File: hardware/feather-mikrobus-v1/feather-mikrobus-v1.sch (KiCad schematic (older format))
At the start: 25 parts, among them J1 Adafruit_Feather_socket_heade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, J2 Adafruit_Feather_socket_heade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, J3 mikroBUS_socket_header_left_p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, J4 mikroBUS_socket_header_right_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, SW1 C_and_K_JS102011SAQN, SW2 C_and_K_KMR421GULCLFS, SW3 C_and_K_KMR421GULCLFS

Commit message: WIP
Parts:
- C1: symbol Flying_Camp_Design:Murata_GRM188R72A104KA35D -> feather-mikrobus-v1-rescue:Murata_GRM188R72A104KA35D-Flying_Camp_Design
- D1, D2: symbol Flying_Camp_Design:Lite-On_LTST-C193KGKT-5A -> feather-mikrobus-v1-rescue:Lite-On_LTST-C193KGKT-5A-Flying_Camp_Design
- FID1, FID2, FID3: symbol Flying_Camp_Design:Fiducial_1mm_Mask2mm -> feather-mikrobus-v1-rescue:Fiducial_1mm_Mask2mm-Flying_Camp_Design
- J1: symbol Flying_Camp_Design:Adafruit_Feather_socket_header_left_pth -> feather-mikrobus-v1-rescue:Adafruit_Feather_socket_header_left_pth-Flying_Camp_Design
- J2: symbol Flying_Camp_Design:Adafruit_Feather_socket_header_right_pth -> feather-mikrobus-v1-rescue:Adafruit_Feather_socket_header_right_pth-Flying_Camp_Design
- J3: symbol Flying_Camp_Design:mikroBUS_socket_header_left_pth -> feather-mikrobus-v1-rescue:mikroBUS_socket_header_left_pth-Flying_Camp_Design
- J4: symbol Flying_Camp_Design:mikroBUS_socket_header_right_pth -> feather-mikrobus-v1-rescue:mikroBUS_socket_header_right_pth-Flying_Camp_Design
- LOGO1: symbol Flying_Camp_Design:mikroBUS-Logo_11.9x4.1mm_SilkScreen -> feather-mikrobus-v1-rescue:mikroBUS-Logo_11.9x4.1mm_SilkScreen-Flying_Camp_Design
- LOGO2: symbol Flying_Camp_Design:Flying_Camp_Design_logo_7.35x11mm_silkscreen -> feather-mikrobus-v1-rescue:Flying_Camp_Design_logo_7.35x11mm_silkscreen-Flying_Camp_Design
- LOGO3: symbol Flying_Camp_Design:Adafruit_Feather_logo_13.87x6.33mm_silkscreen -> feather-mikrobus-v1-rescue:Adafruit_Feather_logo_13.87x6.33mm_silkscreen-Flying_Camp_Design
- MH1: symbol Flying_Camp_Design:Adafruit_Feather_socket_mounting_holes -> feather-mikrobus-v1-rescue:Adafruit_Feather_socket_mounting_holes-Flying_Camp_Design
- R1: symbol Flying_Camp_Design:Yageo_RC0603JR-071KL -> feather-mikrobus-v1-rescue:Yageo_RC0603JR-071KL-Flying_Camp_Design
- R2, R8: symbol Flying_Camp_Design:Yageo_RC0603JR-07330RL -> feather-mikrobus-v1-rescue:Yageo_RC0603JR-07330RL-Flying_Camp_Design
- R3, R4: symbol Flying_Camp_Design:Yageo_RC0603JR-074K7L -> feather-mikrobus-v1-rescue:Yageo_RC0603JR-074K7L-Flying_Camp_Design
- R5: symbol Flying_Camp_Design:Yageo_RC0603JR-070RL -> feather-mikrobus-v1-rescue:Yageo_RC0603JR-070RL-Flying_Camp_Design
- R6: symbol Flying_Camp_Design:Yageo_RC0603JR-0710KL -> feather-mikrobus-v1-rescue:Yageo_RC0603JR-0710KL-Flying_Camp_Design
- R7: symbol Flying_Camp_Design:Yageo_RC0603JR-07100RL -> feather-mikrobus-v1-rescue:Yageo_RC0603JR-07100RL-Flying_Camp_Design
- SW1: symbol Flying_Camp_Design:C_and_K_JS102011SAQN -> feather-mikrobus-v1-rescue:C_and_K_JS102011SAQN-Flying_Camp_Design
- SW2, SW3: symbol Flying_Camp_Design:C_and_K_KMR421GULCLFS -> feather-mikrobus-v1-rescue:C_and_K_KMR421GULCLFS-Flying_Camp_Design
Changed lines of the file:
@@
 3V3_LED_R
 $Comp
-L Flying_Camp_Design:C_and_K_KMR421GULCLFS SW3
+L feather-mikrobus-v1-rescue:C_and_K_KMR421GULCLFS-Flying_Camp_Design SW3
 U 1 1 5E5A44D1
 P 8800 4800
@@
 $EndComp
 $Comp
-L Flying_Camp_Design:Yageo_RC0603JR-074K7L R4
+L feather-mikrobus-v1-rescue:Yageo_RC0603JR-074K7L-Flying_Camp_Design R4
 U 1 1 5E4ACFB9
 P 7500 2800
@@
 $EndComp
 $Comp
-L Flying_Camp_Design:Yageo_RC0603JR-074K7L R3
+L feather-mikrobus-v1-rescue:Yageo_RC0603JR-074K7L-Flying_Camp_Design R3
 U 1 1 5E4AC677
 P 7100 2800
@@
 $EndComp
 $Comp
-L Flying_Camp_Design:C_and_K_JS102011SAQN SW1
+L feather-mikrobus-v1-rescue:C_and_K_JS102011SAQN-Flying_Camp_Design SW1
 U 1 1 5E49923D
 P 8000 2100
@@
 $EndComp
 $Comp
-L Flying_Camp_Design:+3.3V #PWR08
+L feather-mikrobus-v1-rescue:+3.3V-Flying_Camp_Design #PWR08
 U 1 1 5E401342
 P 7500 2600
@@
 $EndComp
 $Comp
-L Flying_Camp_Design:+3.3V #PWR07
+L feather-mikrobus-v1-rescue:+3.3V-Flying_Camp_Design #PWR07
 U 1 1 5E4009E4
 P 7100 2600
@@
 $EndComp
 $Comp
-L Flying_Camp_Design:+3.3V #PWR02
+L feather-mikrobus-v1-rescue:+3.3V-Flying_Camp_Design #PWR02
 U 1 1 5E3DD319
 P 4800 1300
@@
 $EndComp
 $Comp
-L Flying_Camp_Design:Adafruit_Feather_socket_mounting_holes MH1
+L feather-mikrobus-v1-rescue:Adafruit_Feather_socket_mounting_holes-Flying_Camp_Design MH1
 U 1 1 5E3B84FB
 P 5600 1700
@@
 $EndComp
 $Comp
-L Flying_Camp_Design:Adafruit_Feather_socket_header_left_pth J1
+L feather-mikrobus-v1-rescue:Adafruit_Feather_socket_header_left_pth-Flying_Camp_Design J1
 U 1 1 5E3B727D
 P 5200 2300
@@
 $EndComp
 $Comp
-L Flying_Camp_Design:Adafruit_Feather_socket_header_right_pth J2
+L feather-mikrobus-v1-rescue:Adafruit_Feather_socket_header_right_pth-Flying_Camp_Design J2
 U 1 1 5E3B67CD
 P 5600 2500
@@
 $EndComp
 $Comp
-L Flying_Camp_Design:Adafruit_Feather_logo_13.87x6.33mm_silkscreen LOGO3
+L feather-mikrobus-v1-rescue:Adafruit_Feather_logo_13.87x6.33mm_silkscreen-Flying_Camp_Design LOGO3
 U 1 1 5E42FCDA
 P 5400 1300
@@
 $EndComp
 $Comp
-L Flying_Camp_Design:C_and_K_KMR421GULCLFS SW2
+L feather-mikrobus-v1-rescue:C_and_K_KMR421GULCLFS-Flying_Camp_Design SW2
 U 1 1 5E4768B4
 P 2900 2600
@@
 $EndComp
 $Comp
-L Flying_Camp_Design:+3.3V #PWR0103
+L feather-mikrobus-v1-rescue:+3.3V-Flying_Camp_Design #PWR0103
 U 1 1 5E47840A
 P 2900 1800
@@
 $EndComp
 $Comp
-L Flying_Camp_Design:Yageo_RC0603JR-070RL R5
+L feather-mikrobus-v1-rescue:Yageo_RC0603JR-070RL-Flying_Camp_Design R5
 U 1 1 5E4BAA63
 P 3900 1600
@@
 $EndComp
 $Comp
-L Flying_Camp_Design:Yageo_RC0603JR-071KL R1
+L feather-mikrobus-v1-rescue:Yageo_RC0603JR-071KL-Flying_Camp_Design R1
 U 1 1 5E4237BC
 P 2900 2000
@@
 $EndComp
 $Comp
-L Flying_Camp_Design:Yageo_RC0603JR-07100RL R7
+L feather-mikrobus-v1-rescue:Yageo_RC0603JR-07100RL-Flying_Camp_Design R7
 U 1 1 5E42A109
 P 8700 2400
@@
 $EndComp
 $Comp
-L Flying_Camp_Design:+3.3V #PWR09
+L feather-mikrobus-v1-rescue:+3.3V-Flying_Camp_Design #PWR09
 U 1 1 5E3DE1B7
 P 2100 4600
@@
 $EndComp
 $Comp
-L Flying_Camp_Design:mikroBUS_socket_header_left_pth J3
+L feather-mikrobus-v1-rescue:mikroBUS_socket_header_left_pth-Flying_Camp_Design J3
 U 1 1 5E3C6EE3
 P 2500 5000
@@
 $EndComp
 $Comp
-L Flying_Camp_Design:mikroBUS_socket_header_right_pth J4
+L feather-mikrobus-v1-rescue:mikroBUS_socket_header_right_pth-Flying_Camp_Design J4
 U 1 1 5E3C7996
 P 2900 5000
@@
 $EndComp
 $Comp
-L Flying_Camp_Design:mikroBUS-Logo_11.9x4.1mm_SilkScreen LOGO1
+L feather-mikrobus-v1-rescue:mikroBUS-Logo_11.9x4.1mm_SilkScreen-Flying_Camp_Design LOGO1
 U 1 1 5E3FB24F
 P 2700 4400
@@
 $EndComp
 $Comp
-L Flying_Camp_Design:+3.3V #PWR0107
+L feather-mikrobus-v1-rescue:+3.3V-Flying_Camp_Design #PWR0107
 U 1 1 5E5B7B5B
 P 7900 4500
@@
 $EndComp
 $Comp
-L Flying_Camp_Design:Yageo_RC0603JR-0710KL R6
+L feather-mikrobus-v1-rescue:Yageo_RC0603JR-0710KL-Flying_Camp_Design R6
 U 1 1 5E425364
 P 7900 4700
@@
 $EndComp
 $Comp
-L Flying_Camp_Design:Murata_GRM188R72A104KA35D C1
+L feather-mikrobus-v1-rescue:Murata_GRM188R72A104KA35D-Flying_Camp_Design C1
 U 1 1 5E427A0D
 P 7900 5100
@@
 $EndComp
 $Comp
-L Flying_Camp_Design:Yageo_RC0603JR-07330RL R8
+L feather-mikrobus-v1-rescue:Yageo_RC0603JR-07330RL-Flying_Camp_Design R8
 U 1 1 5E49B00C
 P 6000 4700
@@
 $EndComp
 $Comp
-L Flying_Camp_Design:+3.3V #PWR0110
+L feather-mikrobus-v1-rescue:+3.3V-Flying_Camp_Design #PWR0110
 U 1 1 5E49AFEA
 P 6000 4500
@@
 $EndComp
 $Comp
-L Flying_Camp_Design:Yageo_RC0603JR-07330RL R2
+L feather-mikrobus-v1-rescue:Yageo_RC0603JR-07330RL-Flying_Camp_Design R2
 U 1 1 5E41F1AC
 P 5300 4700
@@
 $EndComp
 $Comp
-L Flying_Camp_Design:+3.3V #PWR0109
+L feather-mikrobus-v1-rescue:+3.3V-Flying_Camp_Design #PWR0109
 U 1 1 5E6244BC
 P 5300 4500
@@
 $EndComp
 $Comp
-L Flying_Camp_Design:Fiducial_1mm_Mask2mm FID3
+L feather-mikrobus-v1-rescue:Fiducial_1mm_Mask2mm-Flying_Camp_Design FID3
 U 1 1 5E3F3D03
 P 4700 7700
@@
 $EndComp
 $Comp
-L Flying_Camp_Design:Fiducial_1mm_Mask2mm FID2
+L feather-mikrobus-v1-rescue:Fiducial_1mm_Mask2mm-Flying_Camp_Design FID2
 U 1 1 5E3F3A33
 P 4700 7500
@@
 $EndComp
 $Comp
-L Flying_Camp_Design:Fiducial_1mm_Mask2mm FID1
+L feather-mikrobus-v1-rescue:Fiducial_1mm_Mask2mm-Flying_Camp_Design FID1
 U 1 1 5E3F32FE
 P 4700 7300
@@
 $EndComp
 $Comp
-L Flying_Camp_Design:Lite-On_LTST-C193KGKT-5A D1
+L feather-mikrobus-v1-rescue:Lite-On_LTST-C193KGKT-5A-Flying_Camp_Design D1
 U 1 1 5E68E113
 P 5300 5600
@@
 $EndComp
 $Comp
-L Flying_Camp_Design:Lite-On_LTST-C193KGKT-5A D2
+L feather-mikrobus-v1-rescue:Lite-On_LTST-C193KGKT-5A-Flying_Camp_Design D2
 U 1 1 5E68EC6D
 P 6000 5600
@@
 $EndComp
 $Comp
-L Flying_Camp_Design:Flying_Camp_Design_logo_7.35x11mm_silkscreen LOGO2
+L feather-mikrobus-v1-rescue:Flying_Camp_Design_logo_7.35x11mm_silkscreen-Flying_Camp_Design LOGO2
 U 1 1 5E6E903B
 P 1200 7300

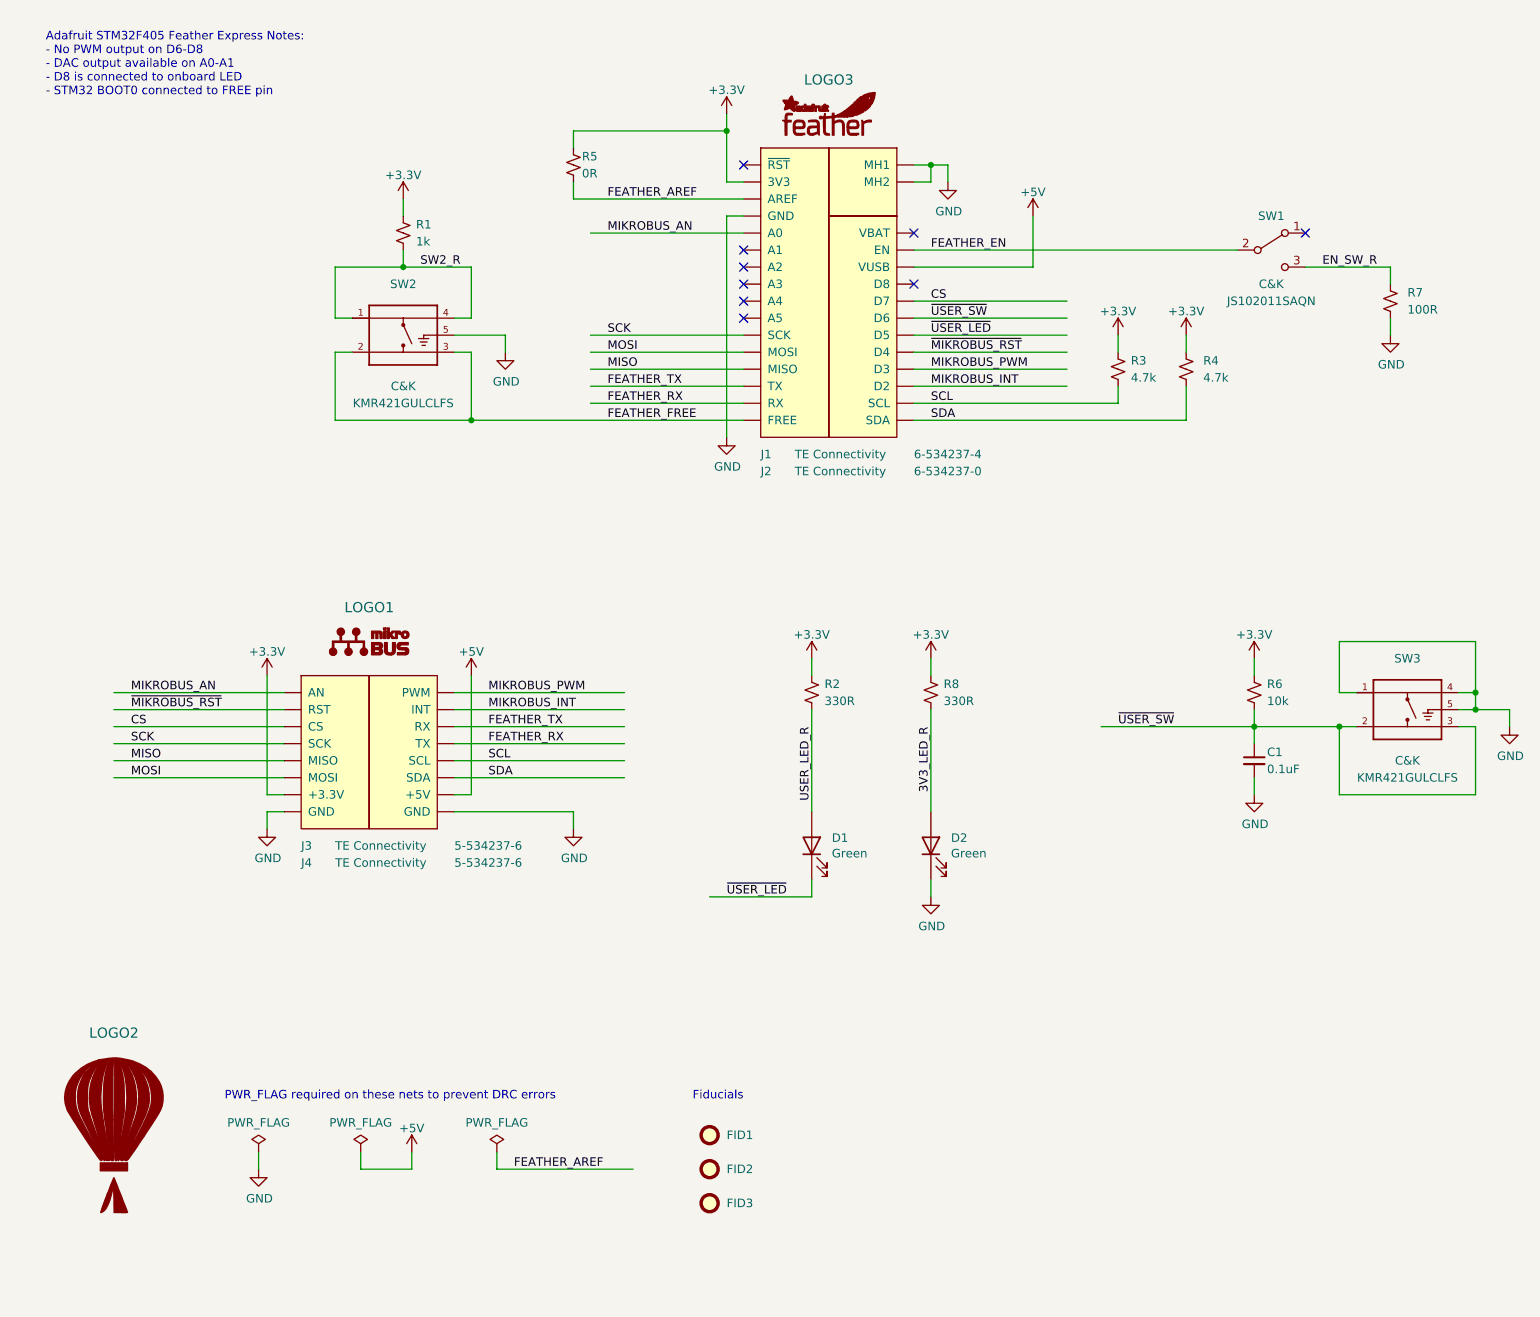
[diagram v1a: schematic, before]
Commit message: [WIP] Update logos
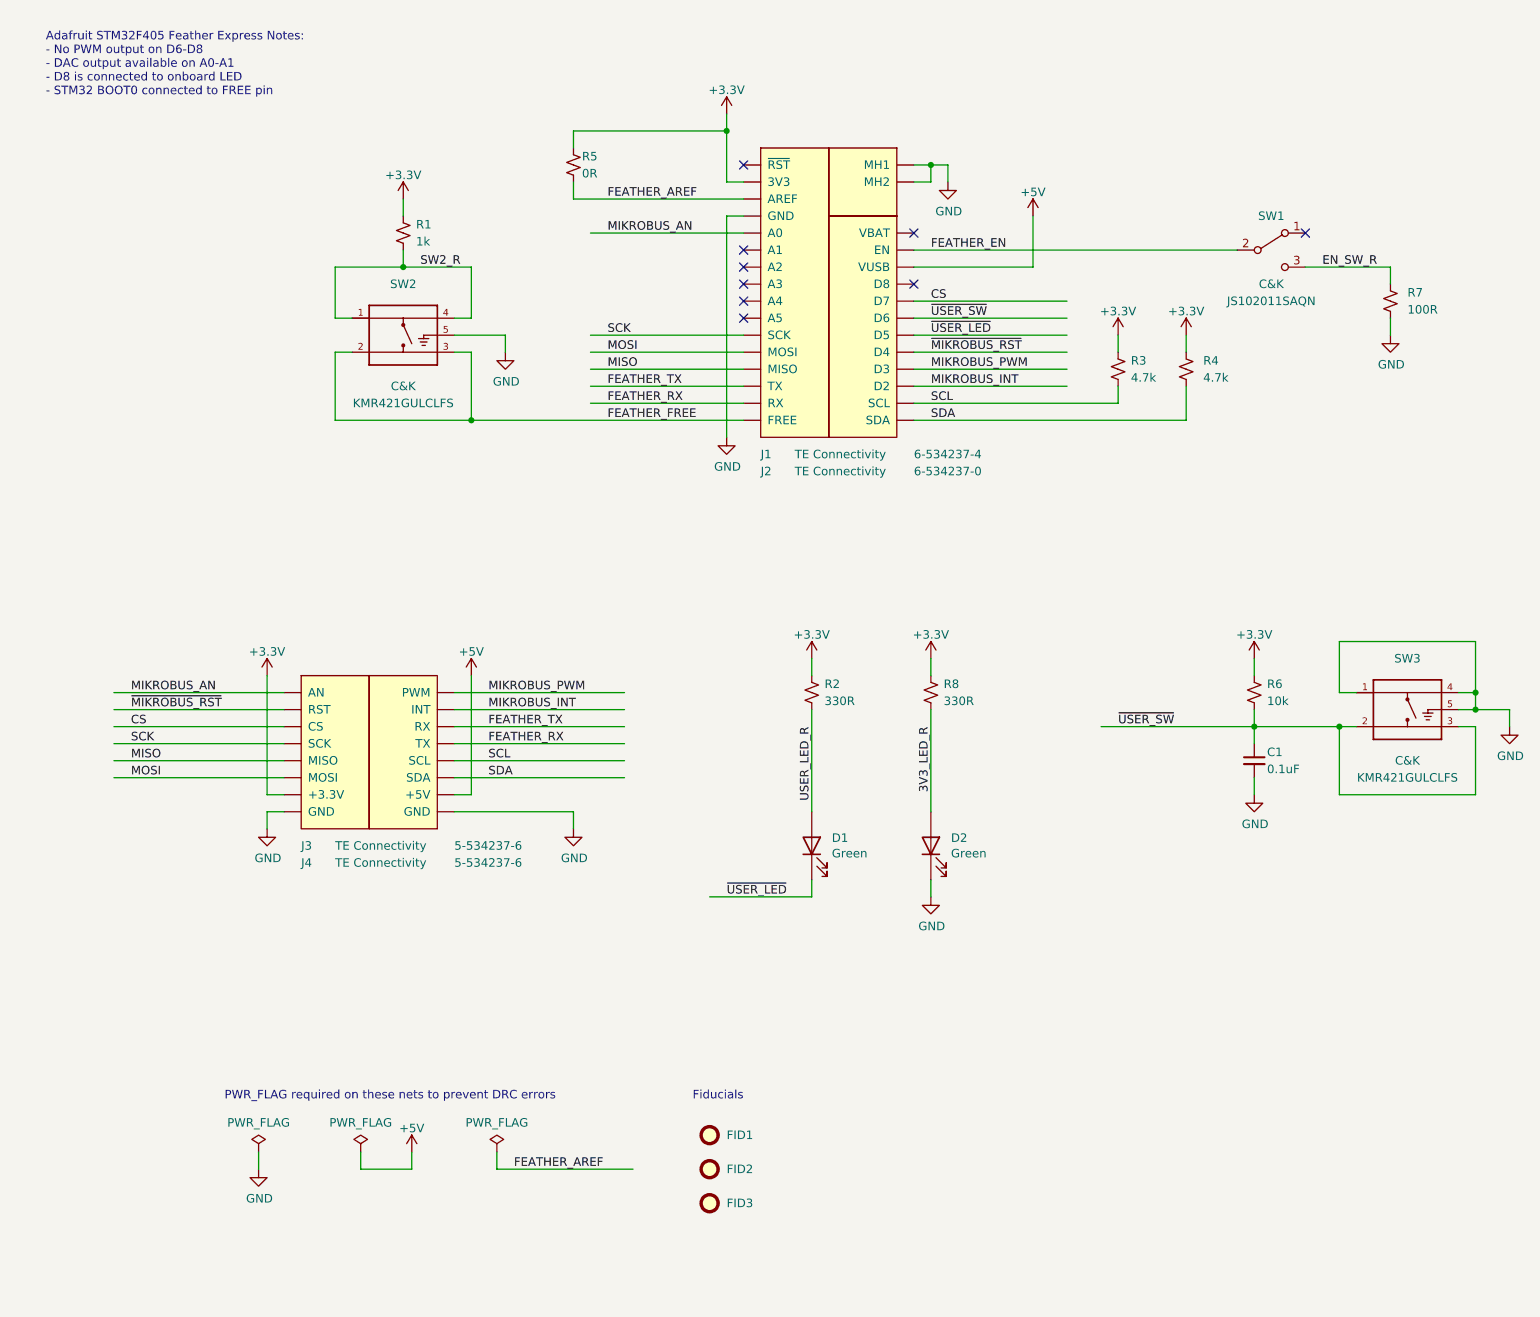
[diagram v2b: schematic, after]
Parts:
- removed LOGO1: mikroBUS-Logo_11.9x4.1mm_SilkScreen, Flying_Camp_Design:mikroBUS-Logo_11.9x4.1mm_SilkScreen, symbol feather-mikrobus-v1-rescue:mikroBUS-Logo_11.9x4.1mm_SilkScreen-Flying_Camp_Desi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
- removed LOGO2: Flying_Camp_Design_logo_7.35x11mm_silkscreen, Flying_Camp_Design:Flying_Camp_Design_logo_7.35x11mm_silkscreen, symbol feather-mikrobus-v1-rescue:Flying_Camp_Design_logo_7.35x11mm_silkscreen-Flying_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
- removed LOGO3: Adafruit_Feather_logo_13.87x6.33mm_silkscreen, Flying_Camp_Design:Adafruit_Feather_logo_13.87x6.33mm_silkscreen, symbol feather-mikrobus-v1-rescue:Adafruit_Feather_logo_13.87x6.33mm_silkscreen-Flying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
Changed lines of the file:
@@
-$EndComp
-$Comp
-L feather-mikrobus-v1-rescue:Adafruit_Feather_logo_13.87x6.33mm_silkscreen-Flying_Camp_Design LOGO3
-U 1 1 5E42FCDA
-P 5400 1300
-F 0 "LOGO3" H 5400 1500 60  0000 C CNN
-F 1 "Adafruit_Feather_logo_13.87x6.33mm_silkscreen" H 5400 1100 50  0001 C CNN
-F 2 "Flying_Camp_Design:Adafruit_Feather_logo_13.87x6.33mm_silkscreen" H 5400 1000 50  0001 C CNN
-F 3 "https://learn.adafruit.com/adafruit-feather/feather-specification" H 5400 900 50  0001 C CNN
-	1    5400 1300
-	1    0    0    -1
 $EndComp
 $Comp
@@
 F 8 "https://www.digikey.com/short/z8mbmb" H 200 100 50  0001 C CNN "Vendor URL"
 	1    2900 5000
-	1    0    0    -1
-$EndComp
-$Comp
-L feather-mikrobus-v1-rescue:mikroBUS-Logo_11.9x4.1mm_SilkScreen-Flying_Camp_Design LOGO1
-U 1 1 5E3FB24F
-P 2700 4400
-F 0 "LOGO1" H 2700 4600 60  0000 C CNN
-F 1 "mikroBUS-Logo_11.9x4.1mm_SilkScreen" H 2700 4200 50  0001 C CNN
-F 2 "Flying_Camp_Design:mikroBUS-Logo_11.9x4.1mm_SilkScreen" H 2700 4100 50  0001 C CNN
-F 3 "https://www.mikroe.com/mikrobus" H 2700 4000 50  0001 C CNN
-	1    2700 4400
 	1    0    0    -1
 $EndComp
@@
 	1    0    0    -1
 $EndComp
-$Comp
-L feather-mikrobus-v1-rescue:Flying_Camp_Design_logo_7.35x11mm_silkscreen-Flying_Camp_Design LOGO2
-U 1 1 5E6E903B
-P 1200 7300
-F 0 "LOGO2" H 1200 7900 60  0000 C CNN
-F 1 "Flying_Camp_Design_logo_7.35x11mm_silkscreen" H 1200 7870 60  0001 C CNN
-F 2 "Flying_Camp_Design:Flying_Camp_Design_logo_7.35x11mm_silkscreen" H 1200 7300 50  0001 C CNN
-F 3 "~" H 1200 7300 50  0001 C CNN
-	1    1200 7300
-	1    0    0    -1
-$EndComp

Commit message: [WIP] Start migration of legacy parts
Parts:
- C1: value Murata_GRM188R72A104KA35D -> Murata_GRM188R72A104KA35D-Flying_Camp_Design
- D1, D2: value Lite-On_LTST-C193KGKT-5A -> Lite-On_LTST-C193KGKT-5A-Flying_Camp_Design
- FID1, FID2, FID3: value Fiducial_1mm_Mask2mm -> FIDUCIAL_GLOBAL_1X2MM; footprint Flying_Camp_Design:Fiducial_1mm_Mask2mm -> Flying_Camp_Design:FIDUCIAL_GLOBAL_1X2MM; symbol feather-mikrobus-v1-rescue:Fiducial_1mm_Mask2mm-Flying_Camp_Design -> Flying_Camp_Design:FIDUCIAL_GLOBAL_1X2MM
- J1: value Adafruit_Feather_socket_header_left_pth -> Adafruit_Feather_socket_header_left_pth-Flying_Camp_Design
- J2: value Adafruit_Feather_socket_header_right_pth -> Adafruit_Feather_socket_header_right_pth-Flying_Camp_Design
- J3: value mikroBUS_socket_header_left_pth -> mikroBUS_socket_header_left_pth-Flying_Camp_Design
- J4: value mikroBUS_socket_header_right_pth -> mikroBUS_socket_header_right_pth-Flying_Camp_Design
- MH1: value Adafruit_Feather_socket_mounting_holes -> Adafruit_Feather_socket_mounting_holes-Flying_Camp_Design
- R1: value Yageo_RC0603JR-071KL -> Yageo_RC0603JR-071KL-Flying_Camp_Design
- R2, R8: value Yageo_RC0603JR-07330RL -> Yageo_RC0603JR-07330RL-Flying_Camp_Design
- R3, R4: value Yageo_RC0603JR-074K7L -> Yageo_RC0603JR-074K7L-Flying_Camp_Design
- R5: value Yageo_RC0603JR-070RL -> Yageo_RC0603JR-070RL-Flying_Camp_Design
- R6: value Yageo_RC0603JR-0710KL -> Yageo_RC0603JR-0710KL-Flying_Camp_Design
- R7: value Yageo_RC0603JR-07100RL -> Yageo_RC0603JR-07100RL-Flying_Camp_Design
- SW1: value C_and_K_JS102011SAQN -> FCD-000051; footprint Flying_Camp_Design:C_and_K_JS102011SAQN -> Flying_Camp_Design:CK_JS102011SAQN; symbol feather-mikrobus-v1-rescue:C_and_K_JS102011SAQN-Flying_Camp_Design -> Flying_Camp_Design:FCD-000051; Part Number (none) -> JS102011SAQN; Vendor Digi-Key -> (none); Vendor Part Number 401-1999-1-ND -> (none); Vendor URL https://www.digikey.com/short/z3mdnv -> (none)
- SW2, SW3: value C_and_K_KMR421GULCLFS -> FCD-000049; footprint Flying_Camp_Design:C_and_K_KMR421GULCLFS -> Flying_Camp_Design:CK_KMR4; symbol feather-mikrobus-v1-rescue:C_and_K_KMR421GULCLFS-Flying_Camp_Design -> Flying_Camp_Design:FCD-000049; Part Number (none) -> KMR421GULCLFS; Vendor Digi-Key -> (none); Vendor Part Number CKN12152CT-ND -> (none); Vendor URL https://www.digikey.com/short/ztqvzm -> (none)
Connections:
- net labels added: +3V3
- net labels removed: +3.3V
